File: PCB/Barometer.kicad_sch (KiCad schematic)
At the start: 1 part, among them U4 BMP280

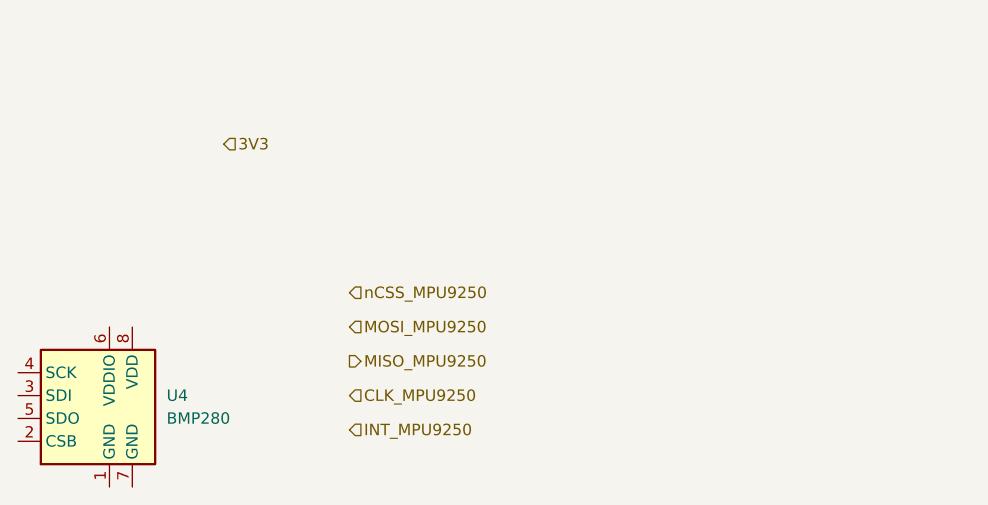
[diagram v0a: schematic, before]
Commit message: Updated PCB
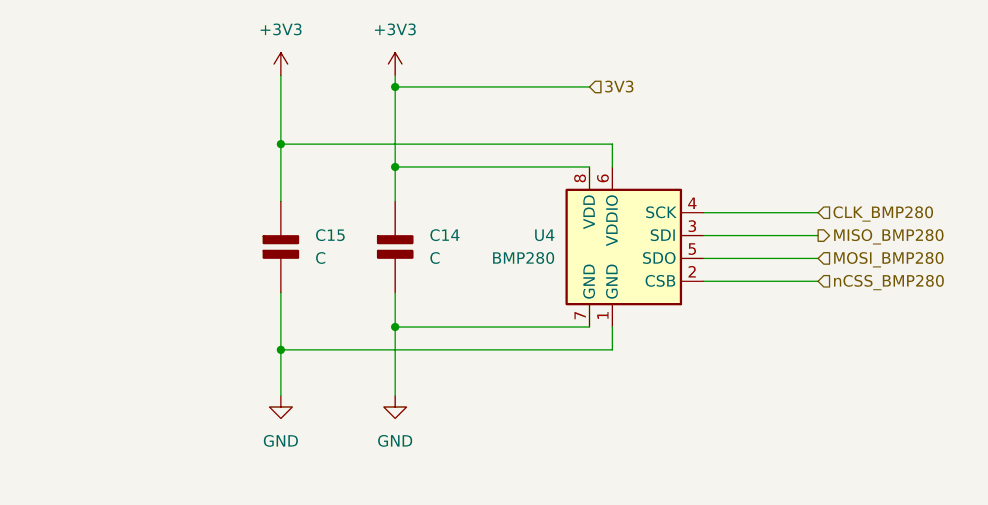
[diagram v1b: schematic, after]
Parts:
- added C14, C15: C, symbol PCM_Elektuur:C
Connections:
- net GND: now reaches U4.1 (GND)
- net GND: now also U4.7 (GND), C14.2 (-), C15.2 (-)
- net nCSS_BMP280: now reaches U4.2 (CSB)
- net MISO_BMP280: now reaches U4.3 (SDI)
- net CLK_BMP280: now reaches U4.4 (SCK)
- net MOSI_BMP280: now reaches U4.5 (SDO)
- net +3V3: now reaches U4.6 (VDDIO)
- net +3V3: now also U4.8 (VDD), C14.1 (+), C15.1 (+)
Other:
- moved on the sheet: U4
